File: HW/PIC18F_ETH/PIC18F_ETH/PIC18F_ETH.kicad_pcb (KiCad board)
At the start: 4 copper layers, 160 x 80 mm, 278 parts, among them J2001 Conn_01x06, J3001 Screw_Terminal_01x02, J3002 JST,2.54, J4001 JST,2.54, J4002 JST,2.54, J4003 JST,2.54, J4004 JST,2.54, J4005 JST,2.54, J4006 JST,2.54, J5001 RJ45_LED_ETH_Shielded, J6001 JST,2.54, J6002 JST,2.54, J8001 JST,2.54, J8002 JST,2.54, J8003 JST,2.54, J8004 JST,2.54, J8005 JST,2.54, J8006 JST,2.54, J8007 JST,2.54, J8008 JST,2.54, J8009 JST,2.54, J8010 JST,2.54, J8011 JST,2.54, J8012 JST,2.54, J8013 JST,2.54, J8014 JST,2.54, J8015 JST,2.54, J8016 JST,2.54, J9001 JST,2.54, J9002 JST,2.54, J9003 JST,2.54, J9004 JST,2.54, J9005 JST,2.54, J9006 JST,2.54, J9007 JST,2.54, J9008 JST,2.54, J9009 JST,2.54, J9010 JST,2.54, J9011 JST,2.54, J9012 JST,2.54, J9013 JST,2.54, J9014 JST,2.54, J9015 JST,2.54, J9016 JST,2.54, U2001 93AA46BT-I/OT, U2002 PIC18F67J60T-I, U2003 25Mhz,50ppm, U3001 LMR51610-Q1, U3002 TPS62A01, U4001 MCP23S17-E/ML, U4002 MCP23S17-E/ML, U6001 25Mhz,50ppm, U6002 MCP2515T-E/ML, U6003 ATA6561-GAQW, U9001 TLP241B, U9002 TLP241B, U9003 TLP241B, U9004 TLP241B, U9005 TLP241B, U9006 TLP241B, U9007 TLP241B, U9008 TLP241B, U9009 TLP241B, U9010 TLP241B, U9011 TLP241B, U9012 TLP241B, U9013 TLP241B, U9014 TLP241B, U9015 TLP241B, U9016 TLP241B

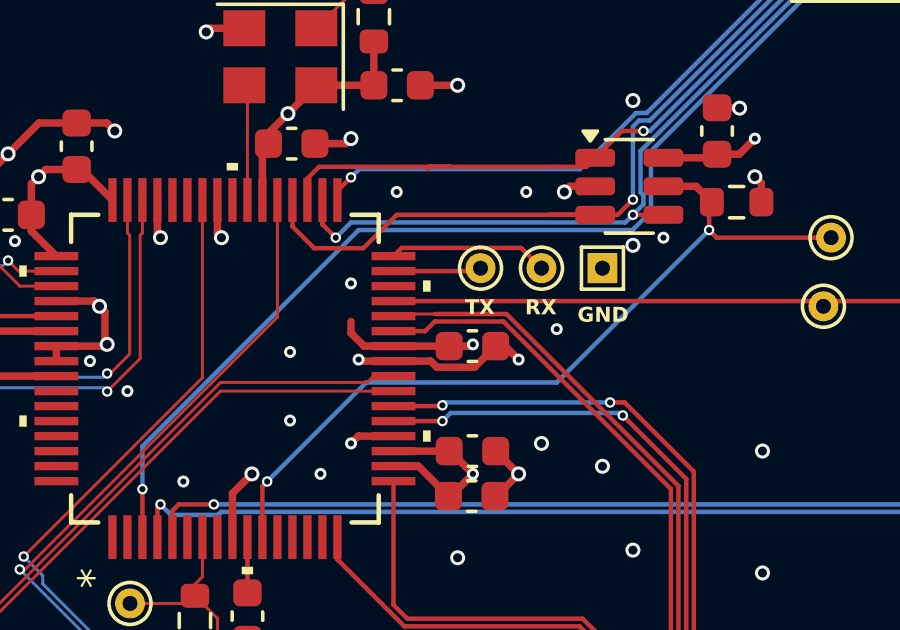
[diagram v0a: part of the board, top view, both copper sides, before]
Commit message: .
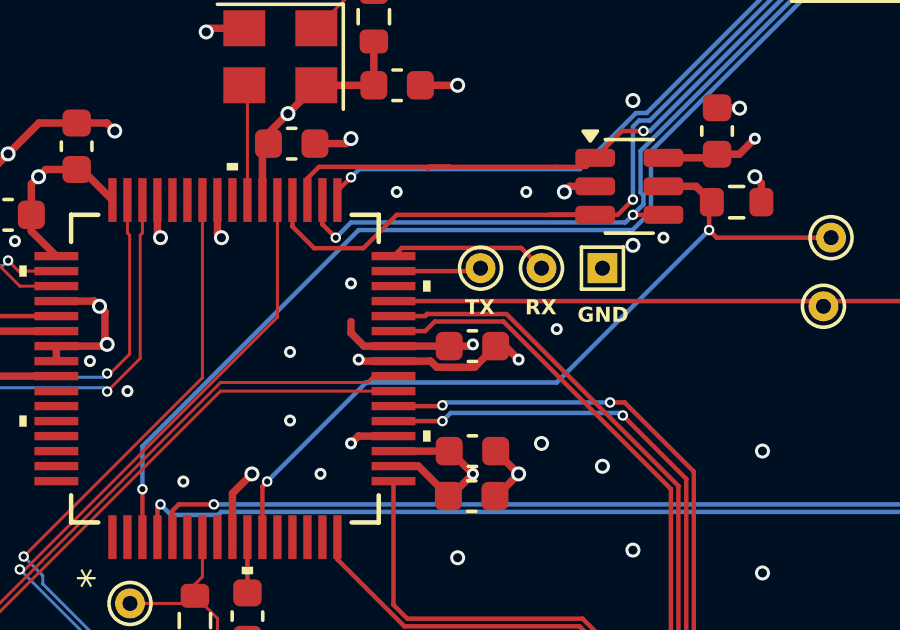
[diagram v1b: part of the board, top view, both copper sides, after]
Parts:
- C3001: value C_Polarized -> 4,7uF 100V
- C3002, C3004, C3006, C3008: value 10u 10V -> 10u 50V
- C3009: value 3n3 50V -> 100n 100V
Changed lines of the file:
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@@
 			)
 		)
-		(property "Value" "10u 10V"
+		(property "Value" "10u 50V"
 			(at 0 1.43 90)
 			(layer "F.Fab")
@@
 			)
 		)
-		(property "CPN" "BT00010-060100"
+		(property "CPN" "BT00007-060100"
 			(at 0 0 90)
 			(unlocked yes)
@@
 			)
 		)
-		(property "Value" "3n3 50V"
+		(property "Value" "100n 100V"
 			(at 0 1.43 90)
 			(layer "F.Fab")
@@
 			)
 		)
-		(property "MPN" "C;C;T1;S;P0603;NA"
+		(property "MPN" "C;M;100n;10p;100V;S;0603"
 			(at 0 0 90)
 			(unlocked yes)
@@
 			)
 		)
-		(property "CPN" "BT00007-090033"
+		(property "CPN" "BT00013-090680"
 			(at 0 0 90)
 			(unlocked yes)
@@
 			)
 		)
-		(property "Value" "10u 10V"
+		(property "Value" "10u 50V"
 			(at 0 1.43 90)
 			(layer "F.Fab")
@@
 			)
 		)
-		(property "CPN" "BT00010-060100"
+		(property "CPN" "BT00007-060100"
 			(at 0 0 90)
 			(unlocked yes)
@@
 			)
 		)
-		(property "Value" "10u 10V"
+		(property "Value" "10u 50V"
 			(at 0 1.43 180)
 			(layer "F.Fab")
@@
 			)
 		)
-		(property "CPN" "BT00010-060100"
+		(property "CPN" "BT00007-060100"
 			(at 0 0 180)
 			(unlocked yes)
@@
 			)
 		)
-		(property "Value" "10u 10V"
+		(property "Value" "10u 50V"
 			(at 0 1.43 0)
 			(layer "F.Fab")
@@
 			)
 		)
-		(property "CPN" "BT00010-060100"
+		(property "CPN" "BT00007-060100"
 			(at 0 0 180)
 			(unlocked yes)
@@
 			)
 		)
-		(property "Value" "C_Polarized"
+		(property "Value" "4,7uF 100V"
 			(at 0 3.2 -90)
 			(layer "F.Fab")
@@
 	)
 	(segment
-		(start 93.688999 138.18)
-		(end 94.996 138.18)
-		(width 0.1)
+		(start 94.742 138.176)
+		(end 94.667999 138.250001)
+		(width 0.15)
 		(layer "F.Cu")
 		(net 5)
 	)
 	(segment
-		(start 97.385554 138.18)
-		(end 94.996 138.18)
+		(start 94.667999 138.250001)
+		(end 93.618998 138.250001)
 		(width 0.15)
 		(layer "F.Cu")
@@
 	)
 	(segment
-		(start 103.116 143.910446)
-		(end 97.385554 138.18)
+		(start 94.746 138.18)
+		(end 94.742 138.176)
 		(width 0.15)
 		(layer "F.Cu")
@@
 	)
 	(segment
-		(start 101.047 159.811)
-		(end 103.116 157.742)
+		(start 101.047 160.528)
+		(end 101.047 159.811)
 		(width 0.15)
 		(layer "F.Cu")
@@
 	)
 	(segment
-		(start 93.618998 138.250001)
-		(end 93.688999 138.18)
-		(width 0.1)
+		(start 97.385554 138.18)
+		(end 94.746 138.18)
+		(width 0.15)
 		(layer "F.Cu")
 		(net 5)
@@
 	)
 	(segment
-		(start 101.047 160.528)
-		(end 101.047 159.811)
+		(start 103.116 143.910446)
+		(end 97.385554 138.18)
+		(width 0.15)
+		(layer "F.Cu")
+		(net 5)
+	)
+	(segment
+		(start 93.618998 138.250001)
+		(end 93.688999 138.18)
+		(width 0.1)
+		(layer "F.Cu")
+		(net 5)
+	)
+	(segment
+		(start 101.047 159.811)
+		(end 103.116 157.742)
 		(width 0.15)
 		(layer "F.Cu")
